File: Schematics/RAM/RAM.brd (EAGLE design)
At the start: 119.4 x 70.8 mm, 17 parts

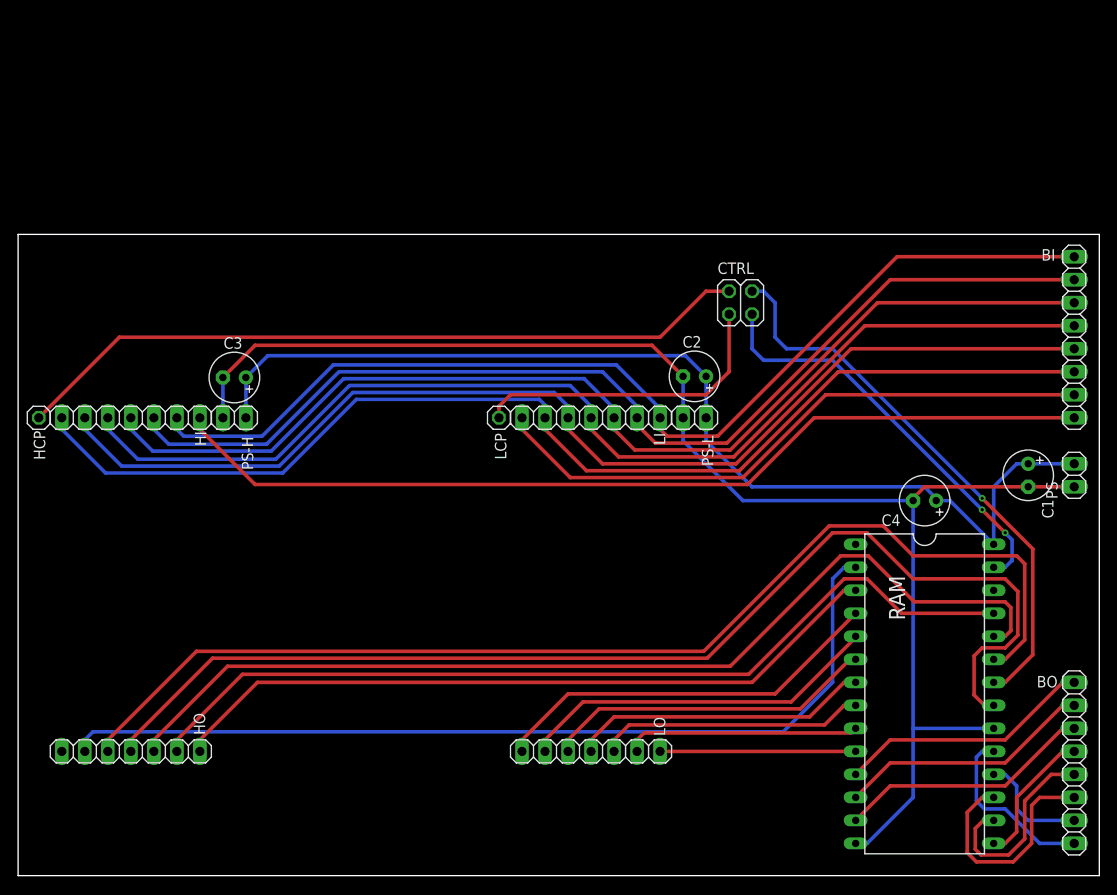
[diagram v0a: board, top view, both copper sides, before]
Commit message: Fixed major mistakes.
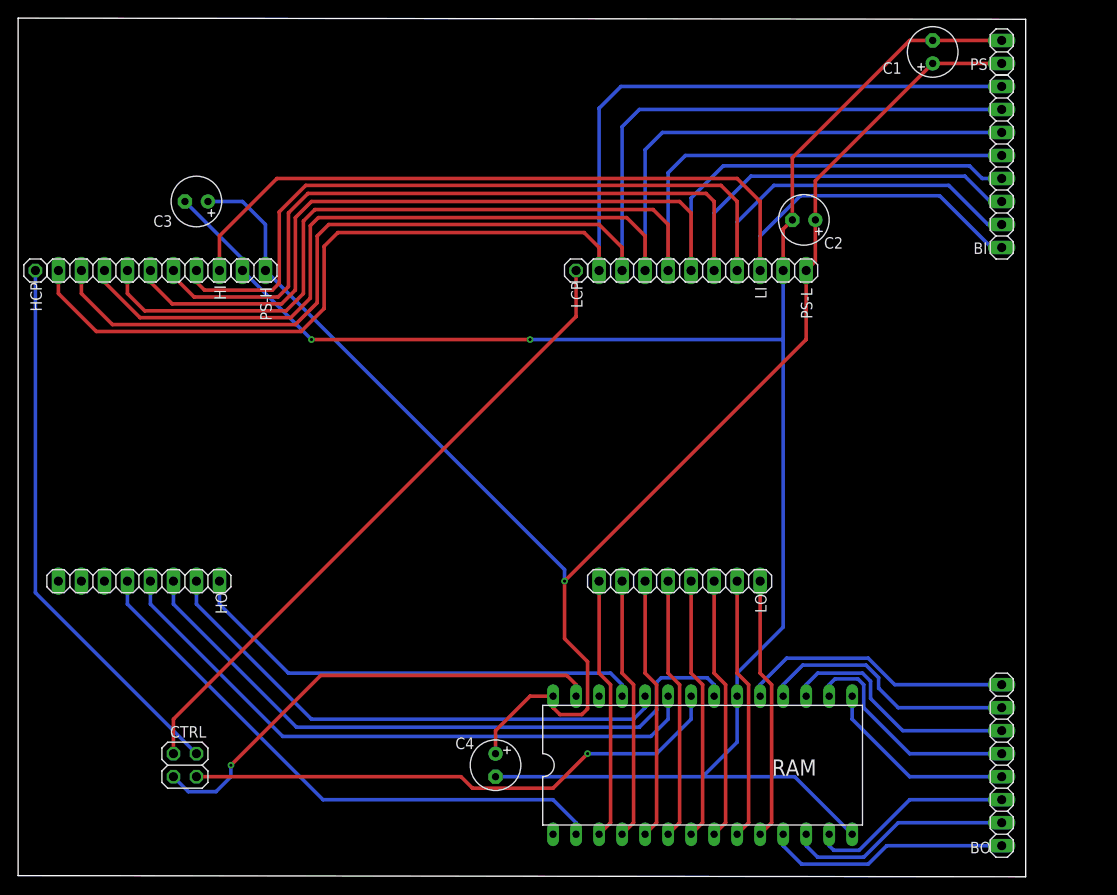
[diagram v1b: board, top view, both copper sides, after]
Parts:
- HI, HO, LI, LO: device pinhead:1X07 -> pinhead:1X08
- moved CTRL 79.8 mm to (18.4, 12.2), turned to 270 degrees
- moved C4 55.7 mm to (52.7, 12.2), turned to 270 degrees
- moved C1 47.9 mm to (101.0, 90.9), turned to 90 degrees
- moved PS 47.4 mm to (108.6, 90.9), turned to 270 degrees
- moved RAM 25.7 mm to (75.6, 12.2), turned to 0 degrees
- moved LO 21.2 mm to (73.0, 32.5)
- moved C2 21.1 mm to (86.7, 72.4)
- moved BI 20.4 mm to (108.6, 78.2), turned to 270 degrees
- moved C3 19.9 mm to (19.7, 74.4)
- moved PS-L 19.7 mm to (85.7, 66.8)
- moved LI 19.0 mm to (73.0, 66.8)
- moved HO 18.8 mm to (13.3, 32.5)
- moved LCP 18.3 mm to (61.6, 66.8)
- moved PS-H 16.4 mm to (26.0, 66.8)
- moved HI 16.3 mm to (13.3, 66.8)
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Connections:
- net A0: now also LO.8; no longer LO.7
- net A1: now also LO.7; no longer LO.6
- net A10: now also HO.6; no longer HO.4
- net A11: now also HO.5; no longer HO.3
- net A12: now also HO.4; no longer HO.2
- net A2: now also LO.6; no longer LO.5
- net A3: now also LO.5; no longer LO.4
- net A4: now also LO.4; no longer LO.3
- net A5: now also LO.3; no longer LO.2
- net A6: now also LO.2; no longer LO.1
- net A7: now also LO.1; no longer HO.7
- net A8: now also HO.8; no longer HO.6
- net A9: now also HO.7; no longer HO.5
- net B0: now also HI.8, LI.8; no longer HI.6, LI.7
- net B1: now also HI.7, LI.7; no longer HI.5, LI.6
- net B2: now also HI.6, LI.6; no longer HI.4, LI.5
- net B3: now also HI.5, LI.5; no longer HI.3, LI.4
- net B4: now also HI.4, LI.4; no longer HI.2, LI.3
- net B5: now also HI.3, LI.3; no longer HI.1, LI.2
- net B6: now also HI.2, LI.2; no longer LI.1
- net B7: now also HI.1, LI.1; no longer HI.7
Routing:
- net B6: track 68.2 -> 134.7 mm
- net A11: track 126.7 -> 69.1 mm
- net VCC: track 117.2 -> 173.3 mm, vias 0 -> 1
- net A10: track 128.9 -> 73.5 mm
- net GND: track 162.1 -> 216.0 mm, vias 0 -> 2
- net A9: track 111.4 -> 59.1 mm
- net A7: track 80.5 -> 29.0 mm
- net A8: track 100.4 -> 51.9 mm
- net A12: track 100.9 -> 63.3 mm
- net LCP: track 34.6 -> 71.8 mm
- net B7: track 103.4 -> 139.1 mm
- net HCP: track 82.0 -> 60.7 mm
- net O6: track 12.5 -> 28.9 mm
- net A6: track 43.9 -> 29.0 mm
- net A5: track 40.4 -> 29.0 mm
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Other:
- board size 119.4 x 70.8 mm -> 111.2 x 94.8 mm
